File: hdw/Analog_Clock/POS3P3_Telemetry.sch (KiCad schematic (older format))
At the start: 7 parts

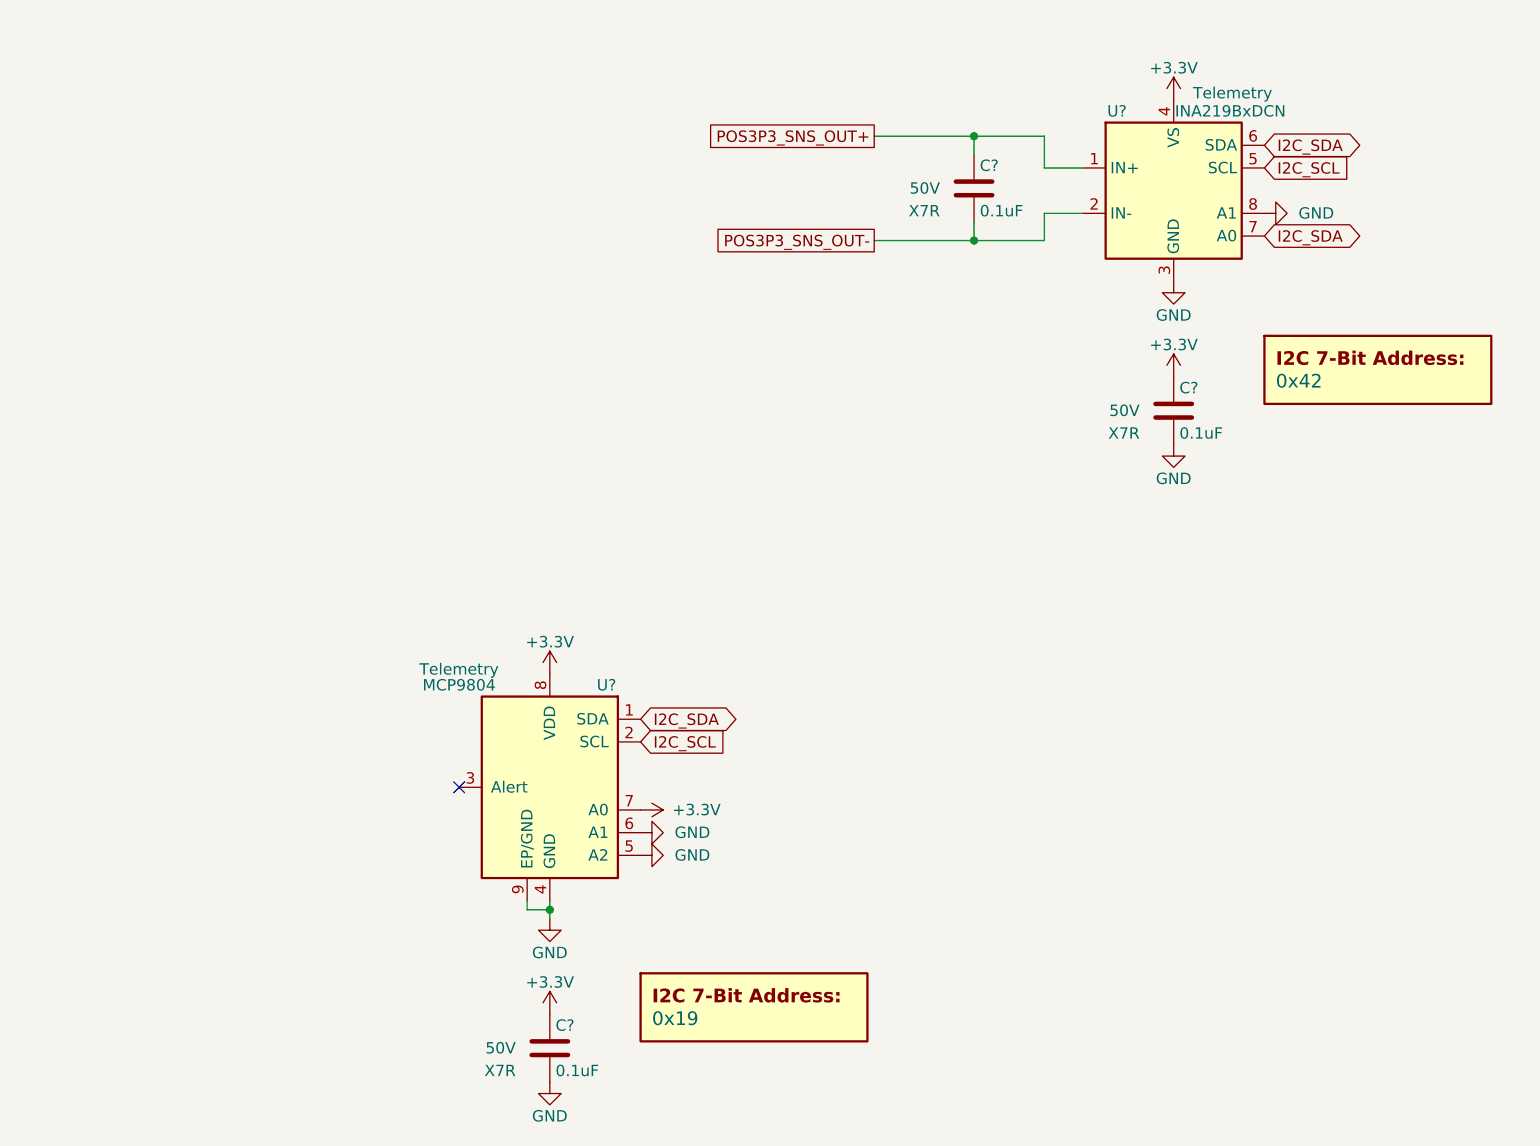
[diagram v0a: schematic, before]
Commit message: More sch work
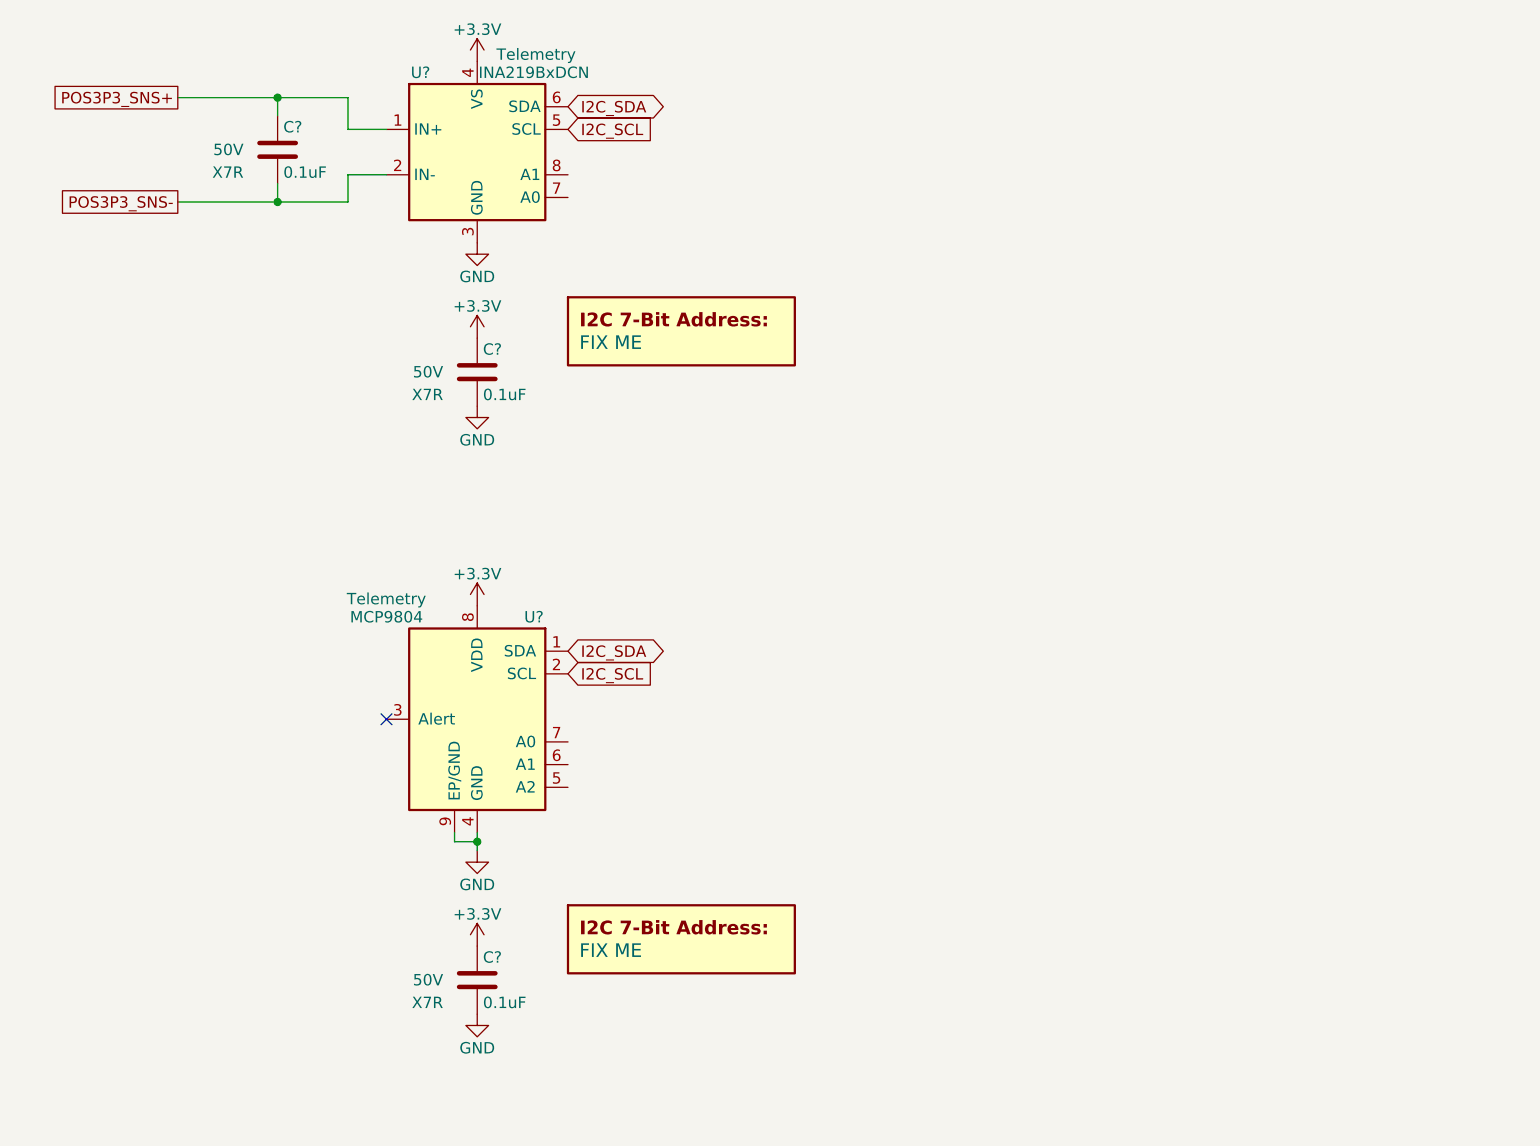
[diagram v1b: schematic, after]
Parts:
- removed C? (x3): 0.1uF, Capacitors_SMD:C_0402, symbol Custom_Library:C_Custom
- removed DOC?: 0x42, symbol Custom_Library:I2C_Address
- removed DOC?: 0x19, symbol Custom_Library:I2C_Address
- removed U?: INA219BxDCN, Package_TO_SOT_SMD:SOT-23-8, symbol Analog_ADC:INA219BxDCN
- removed U?: MCP9804, Package_DFN_QFN:DFN-8-1EP_3x2mm_P0.5mm_EP1.3x1.5mm, symbol Sensor_Temperature:MCP9804_DFN
- added C? (x3): 0.1uF, Capacitors_SMD:C_0402, symbol Custom_Library:C_Custom
- added DOC? (x2): FIX ME, symbol Custom_Library:I2C_Address
- added U?: INA219BxDCN, Package_TO_SOT_SMD:SOT-23-8, symbol Analog_ADC:INA219BxDCN
- added U?: MCP9804, Package_DFN_QFN:DFN-8-1EP_3x2mm_P0.5mm_EP1.3x1.5mm, symbol Sensor_Temperature:MCP9804_DFN
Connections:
- net +3V3: now also C?.1, C?.1, U?.4 (VS), U?.8 (VDD)
- net GND: now also C?.2, C?.2, U?.3 (GND), U?.4 (GND), U?.9 (EP/GND)
- net I2C_SCL: now also U?.2 (SCL), U?.5 (SCL)
- net I2C_SDA: now also U?.1 (SDA), U?.6 (SDA)
- new net POS3P3_SNS+: C?.1, U?.1 (IN+)
- new net POS3P3_SNS-: C?.2, U?.2 (IN-)
